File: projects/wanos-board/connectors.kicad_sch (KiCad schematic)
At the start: 7 parts, among them J2 DOOR_SAUNA, J3 DOOR_BATH, J4 WATER_B1, J5 WATER_B2, J6 KWH_MAIN, J7 KWH_AUX, J8 BTN_SAUNA

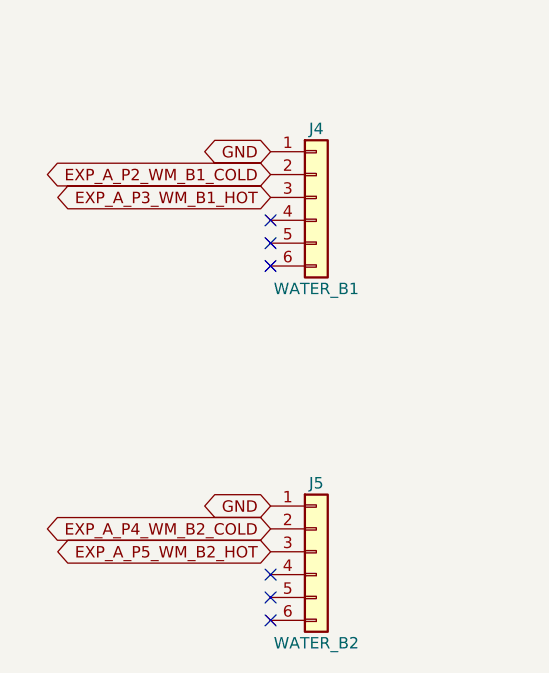
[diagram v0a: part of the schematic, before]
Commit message: 1st draft: water meters schematic
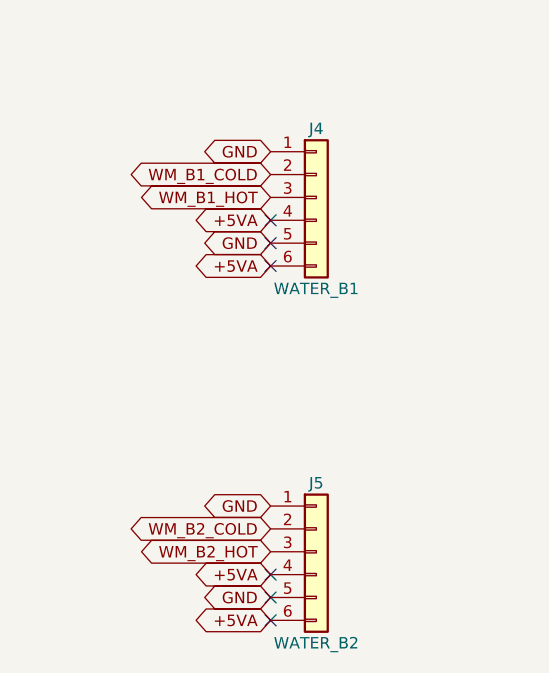
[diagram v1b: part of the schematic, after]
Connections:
- net GND: now also J4.5 (Pin_5), J5.5 (Pin_5)
- net +5VA: now reaches J5.4 (Pin_4)
- net +5VA: now also J4.4 (Pin_4), J4.6 (Pin_6), J5.6 (Pin_6)
- net EXP_A_P2_WM_B1_COLD renamed WM_B1_COLD
- net EXP_A_P3_WM_B1_HOT renamed WM_B1_HOT
- net EXP_A_P4_WM_B2_COLD renamed WM_B2_COLD
- net EXP_A_P5_WM_B2_HOT renamed WM_B2_HOT
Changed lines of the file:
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@@
 		)
 	)
-	(global_label "EXP_A_P4_WM_B2_COLD"
+	(global_label "WM_B2_COLD"
 		(shape bidirectional)
 		(at 25.4 127 180)
@@
 		)
 	)
-	(global_label "EXP_A_P3_WM_B1_HOT"
+	(global_label "WM_B1_HOT"
 		(shape bidirectional)
 		(at 25.4 90.17 180)
@@
 		)
 	)
-	(global_label "EXP_A_P2_WM_B1_COLD"
+	(global_label "WM_B1_COLD"
 		(shape bidirectional)
 		(at 25.4 87.63 180)
@@
 		)
 	)
-	(global_label "EXP_A_P5_WM_B2_HOT"
+	(global_label "WM_B2_HOT"
 		(shape bidirectional)
 		(at 25.4 129.54 180)
@@
 			(hide yes)
 			(show_name no)
+			(do_not_autoplace no)
+			(effects
+				(font
+					(size 1.27 1.27)
+				)
+			)
+		)
+	)
+	(global_label "+5VA"
+		(shape bidirectional)
+		(at 25.4 92.71 180)
+		(effects
+			(font
+				(size 1.27 1.27)
+			)
+			(justify right bottom)
+		)
+		(property "Intersheetrefs" "${INTERSHEET_REFS}"
+			(at 25.4 92.71 0)
+			(hide yes)
+			(show_name no)
+			(do_not_autoplace no)
+			(effects
+				(font
+					(size 1.27 1.27)
+				)
+			)
+		)
+	)
+	(global_label "GND"
+		(shape bidirectional)
+		(at 25.4 95.25 180)
+		(effects
+			(font
+				(size 1.27 1.27)
+			)
+			(justify right bottom)
+		)
+		(property "Intersheetrefs" "${INTERSHEET_REFS}"
+			(at 25.4 95.25 0)
+			(hide yes)
+			(show_name no)
+			(do_not_autoplace no)
+			(effects
+				(font
+					(size 1.27 1.27)
+				)
+			)
+		)
+	)
+	(global_label "+5VA"
+		(shape bidirectional)
+		(at 25.4 97.79 180)
+		(effects
+			(font
+				(size 1.27 1.27)
+			)
+			(justify right bottom)
+		)
+		(property "Intersheetrefs" "${INTERSHEET_REFS}"
+			(at 25.4 97.79 0)
+			(hide yes)
+			(show_name no)
+			(do_not_autoplace no)
+			(effects
+				(font
+					(size 1.27 1.27)
+				)
+			)
+		)
+	)
+	(global_label "+5VA"
+		(shape bidirectional)
+		(at 25.4 132.08 180)
+		(effects
+			(font
+				(size 1.27 1.27)
+			)
+			(justify right bottom)
+		)
+		(property "Intersheetrefs" "${INTERSHEET_REFS}"
+			(at 25.4 132.08 0)
+			(hide yes)
+			(show_name no)
+			(do_not_autoplace no)
+			(effects
+				(font
+					(size 1.27 1.27)
+				)
+			)
+		)
+	)
+	(global_label "GND"
+		(shape bidirectional)
+		(at 25.4 134.62 180)
+		(effects
+			(font
+				(size 1.27 1.27)
+			)
+			(justify right bottom)
+		)
+		(property "Intersheetrefs" "${INTERSHEET_REFS}"
+			(at 25.4 134.62 0)
+			(hide yes)
+			(show_name no)
+			(do_not_autoplace no)
+			(effects
+				(font
+					(size 1.27 1.27)
+				)
+			)
+		)
+	)
+	(global_label "+5VA"
+		(shape bidirectional)
+		(at 25.4 137.16 180)
+		(effects
+			(font
+				(size 1.27 1.27)
+			)
+			(justify right bottom)
+		)
+		(property "Intersheetrefs" "${INTERSHEET_REFS}"
+			(at 25.4 137.16 0)
+			(hide yes)
+			(show_name no)
